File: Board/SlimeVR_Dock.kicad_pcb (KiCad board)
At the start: 2 copper layers, 163.1 x 106 mm, 113 parts, among them J1Fan1 Conn_01x04_Pin, J1Temp1 Conn_01x05_Pin, J1_Control1 Conn_01x03_Pin, J1_MainPW1 USB_C_Receptacle_USB2.0_16P, J1_Monitor1 Conn_01x03_Pin, J1_Prog1 Conn_01x03_Pin, J2 USB_C_Receptacle_USB2.0_16P, J3 USB_C_Receptacle_USB2.0_16P, J4 USB_C_Receptacle_USB2.0_16P, J5 USB_C_Receptacle_USB2.0_16P, J6 USB_C_Receptacle_USB2.0_16P, J7 USB_C_Receptacle_USB2.0_16P, J8 USB_C_Receptacle_USB2.0_16P, J9 USB_C_Receptacle_USB2.0_16P, Q1 NDT452AP, Q2 BC857, Q3 BC857, Q4 BC857, Q5 BC857, Q6 BC817, U1 ESP32-C3-WROOM-02, U10 INA226, U11 AP22652W6-7, U12 INA226, U13 INA226, U14 AP22652W6-7, U15 INA226, U16 INA226, U17 74HC165, U18 74HC165, U19 74HC595, U2 CH224K, U3 XC6220B331MR, U4 TPS548A20RVER, U5 AP22652W6-7, U6 INA226, U7 INA226, U8 AP22652W6-7, U9 INA226

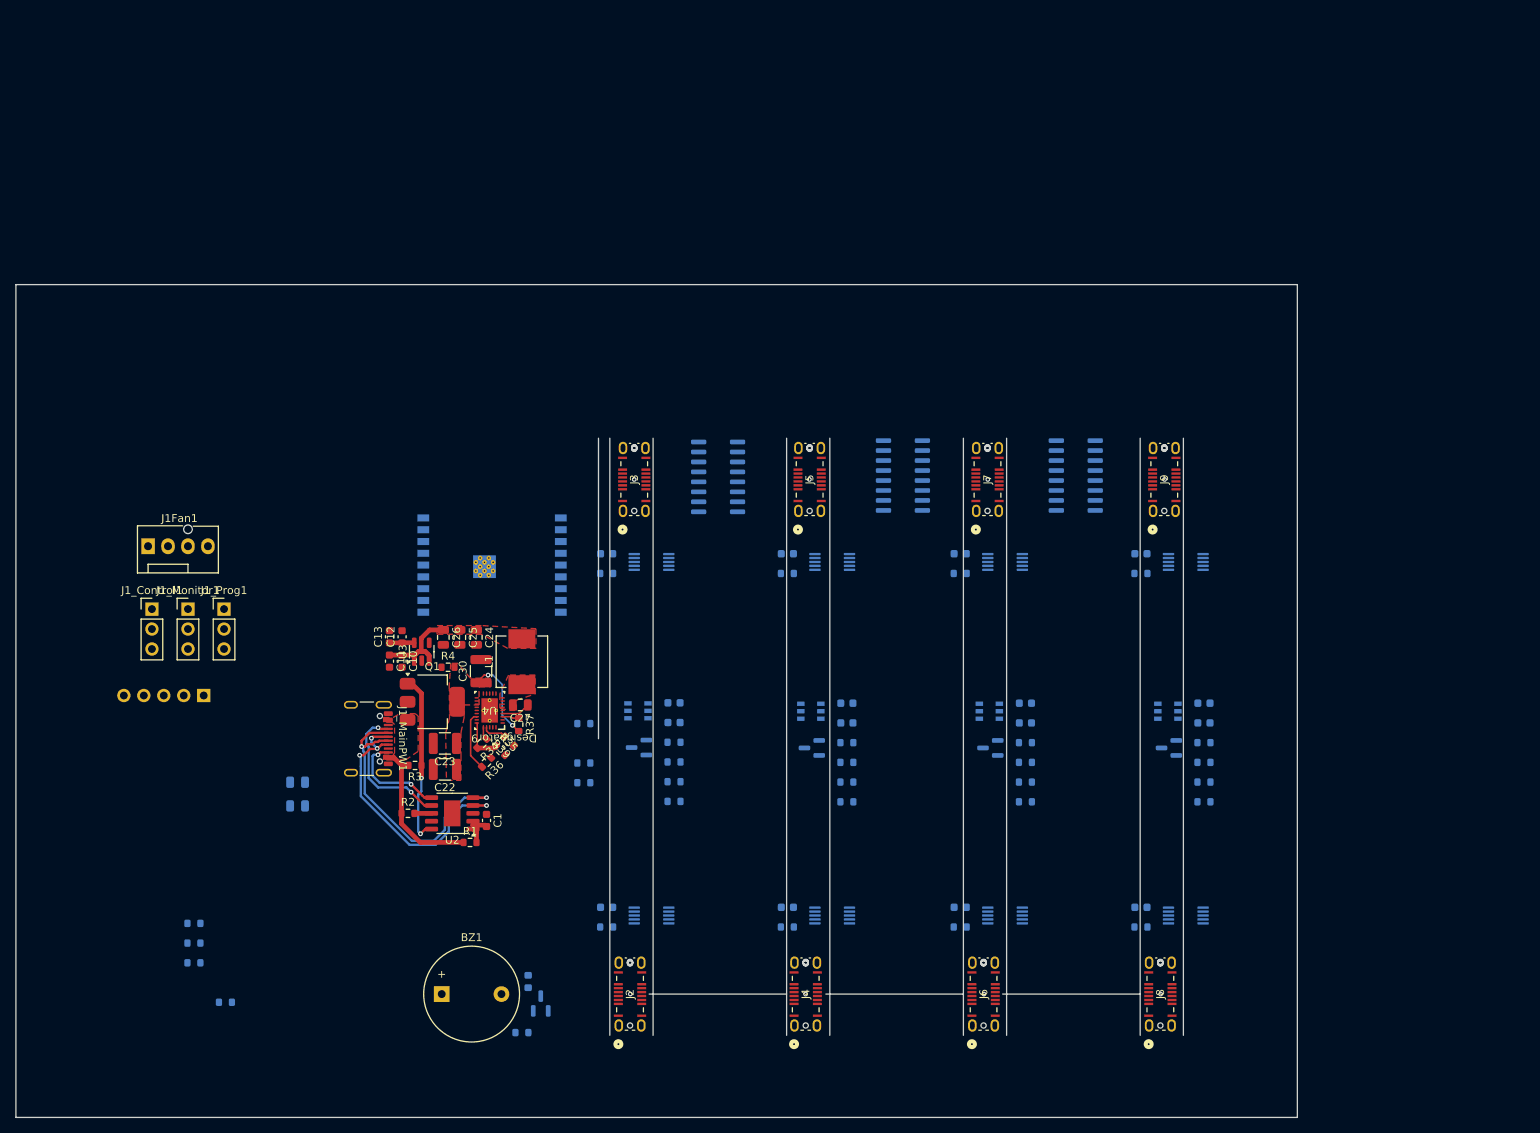
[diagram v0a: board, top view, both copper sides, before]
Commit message: upraveni veliskoti
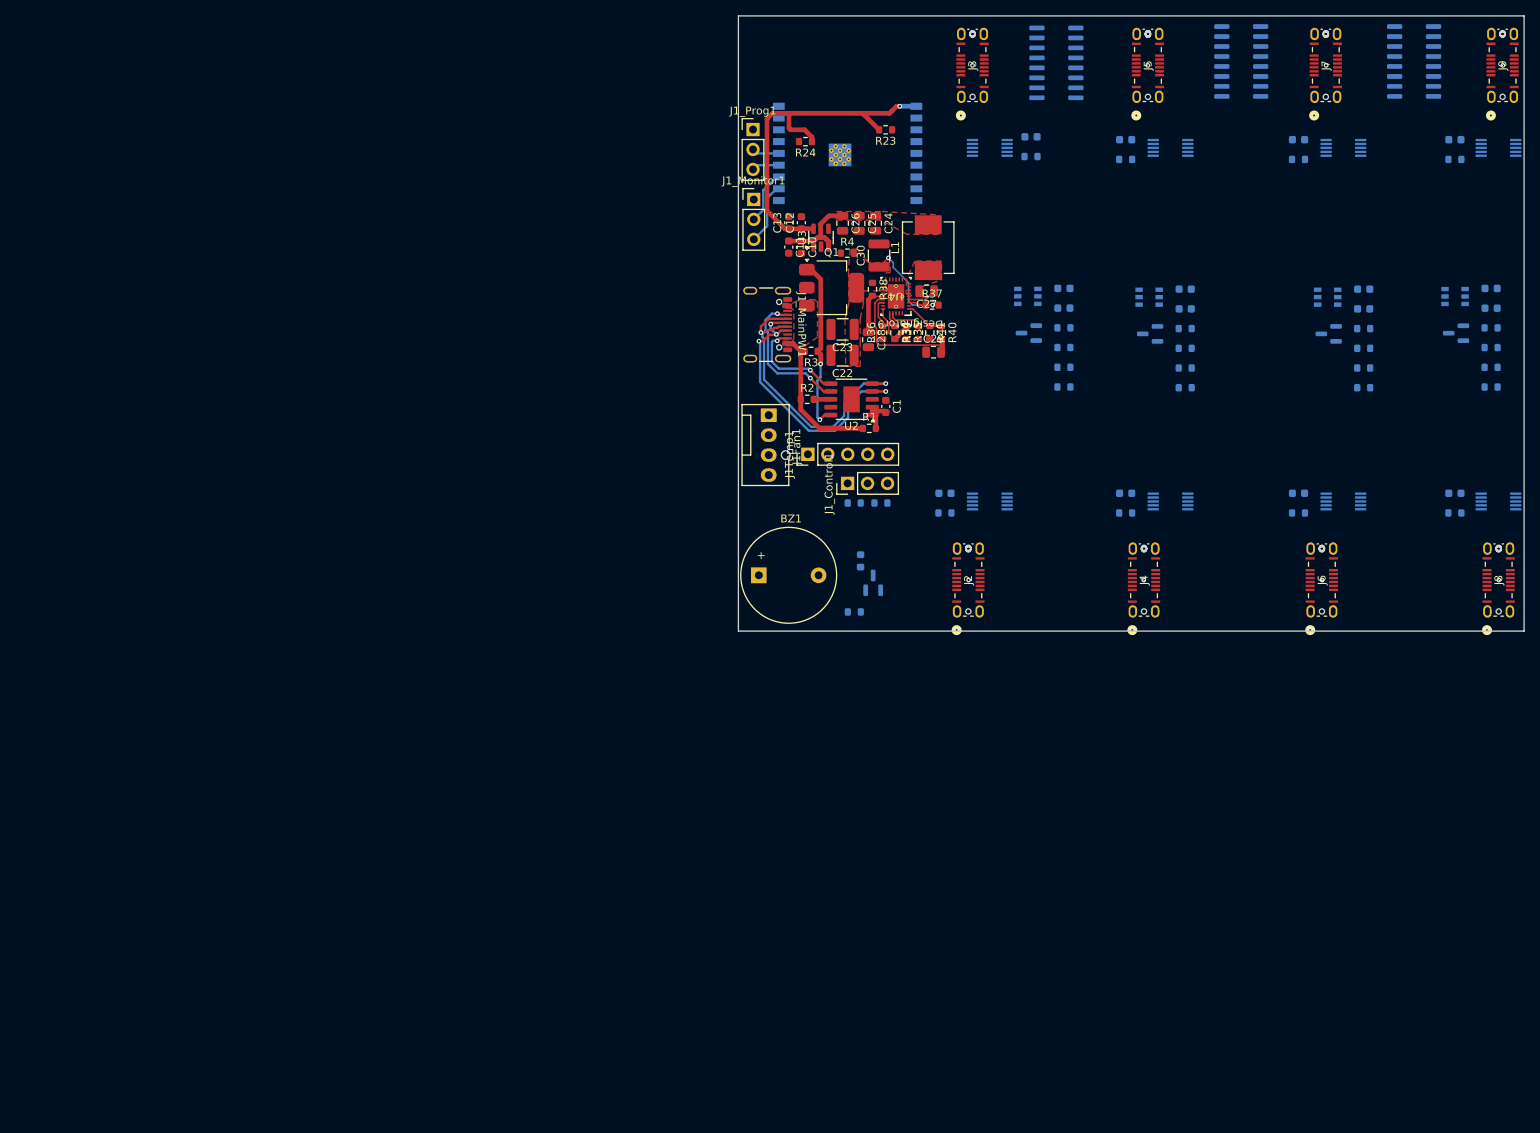
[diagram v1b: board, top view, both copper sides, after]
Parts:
- C28, C29, J1Temp1, R23, R24, R38, R40, R41: moved to F.Cu
- moved R23 135.9 mm to (114.8, 74.0)
- moved R24 130.3 mm to (104.6, 75.5)
- moved R17 104.9 mm to (114.2, 121.5), turned to 0 degrees
- moved R18 99.6 mm to (110.8, 121.5)
- moved C29 99.4 mm to (120.9, 102.3), turned to 0 degrees
- moved C28 91.9 mm to (112.6, 100.7), turned to -90 degrees
- moved J1_Prog1 90.9 mm to (97.9, 74.0)
- moved J1_Control1 90.0 mm to (110.0, 119.0), turned to 90 degrees
- moved J1_Monitor1 88.9 mm to (98.0, 82.9)
- moved J1Temp1 82.8 mm to (104.9, 115.3)
- moved J1Fan1 80.7 mm to (99.9, 110.3), turned to -90 degrees
- moved C15 75.7 mm to (133.3, 74.9)
- moved R26 75.7 mm to (133.3, 77.4)
- moved R37 75.0 mm to (120.7, 96.3), turned to 0 degrees
- moved R36 74.4 mm to (114.4, 99.8), turned to 90 degrees
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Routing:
- net +3V3: track 3.16 -> 47.0 mm, vias 0 -> 1
- net Net-(U4-VREG): track 0.00 -> 17.3 mm
- net RX: track 0.00 -> 7.94 mm
- net TX: track 0.00 -> 6.90 mm
- net Net-(U4-VDD): track 0.00 -> 6.23 mm
- net Net-(U4-RF): track 0.00 -> 5.05 mm
- net Net-(U4-MODE): track 7.57 -> 3.79 mm
- net D-: track 0.00 -> 3.51 mm
- net D+: track 0.00 -> 3.50 mm
- net /StepDown/Vin: track 10.8 -> 12.3 mm
- net Net-(U4-TRIP): track 3.06 -> 4.49 mm
- net Net-(U4-FB): track 5.72 -> 6.72 mm
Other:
- board size 163.1 x 106 mm -> 100 x 78.3 mm
